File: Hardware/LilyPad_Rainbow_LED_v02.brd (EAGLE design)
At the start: 38.6 x 12.7 mm, 37 parts

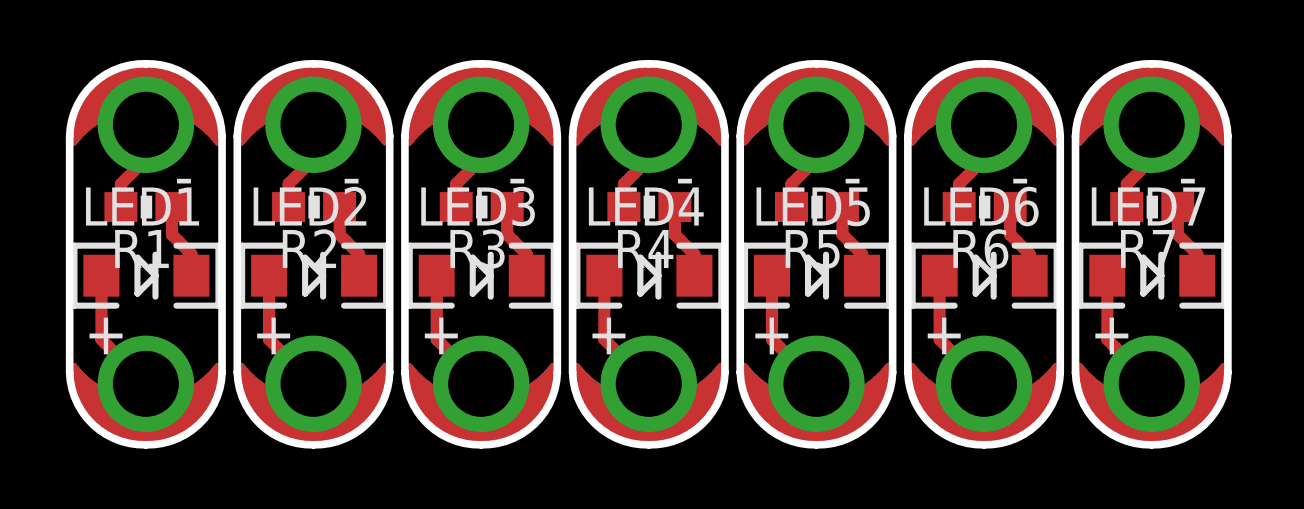
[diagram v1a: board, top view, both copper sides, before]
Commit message: Updated brd file
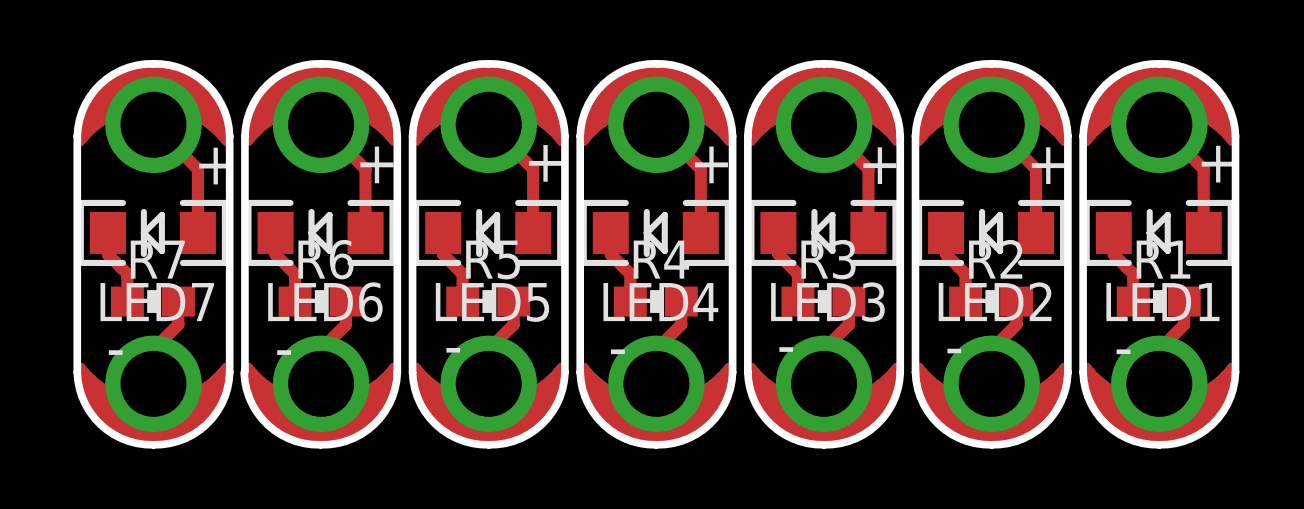
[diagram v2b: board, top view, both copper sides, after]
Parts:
- moved LED+1 34.9 mm to (36.6, 10.0), turned to 180 degrees
- moved LED-1 34.9 mm to (36.6, 1.40), turned to 0 degrees
- moved LED+7 34.4 mm to (3.05, 10.0), turned to 180 degrees
- moved LED-7 34.4 mm to (3.05, 1.40), turned to 0 degrees
- moved R1 33.9 mm to (36.6, 4.14), turned to 0 degrees
- moved LOGO35 33.8 mm to (36.6, 5.44)
- moved LED1 33.8 mm to (36.6, 6.43), turned to 180 degrees
- moved R7 33.5 mm to (3.03, 4.14), turned to 0 degrees
- moved LED7 33.3 mm to (3.03, 6.43), turned to 180 degrees
- moved LOGO30 33.2 mm to (3.12, 5.44)
- moved LED+2 24.2 mm to (31.0, 10.0), turned to 180 degrees
- moved LED-2 24.2 mm to (31.0, 1.40), turned to 0 degrees
- moved LED+6 23.7 mm to (8.64, 10.0), turned to 180 degrees
- moved LED-6 23.7 mm to (8.64, 1.40), turned to 0 degrees
- moved R2 22.8 mm to (31.0, 4.14), turned to 0 degrees
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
